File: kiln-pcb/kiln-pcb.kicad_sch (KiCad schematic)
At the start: 14 parts, among them J1 TFT, J2 TEMP, J3 ROTARY, J4 Relay, J5 Relay, J6 Relay, U1 WeMos_D1_mini

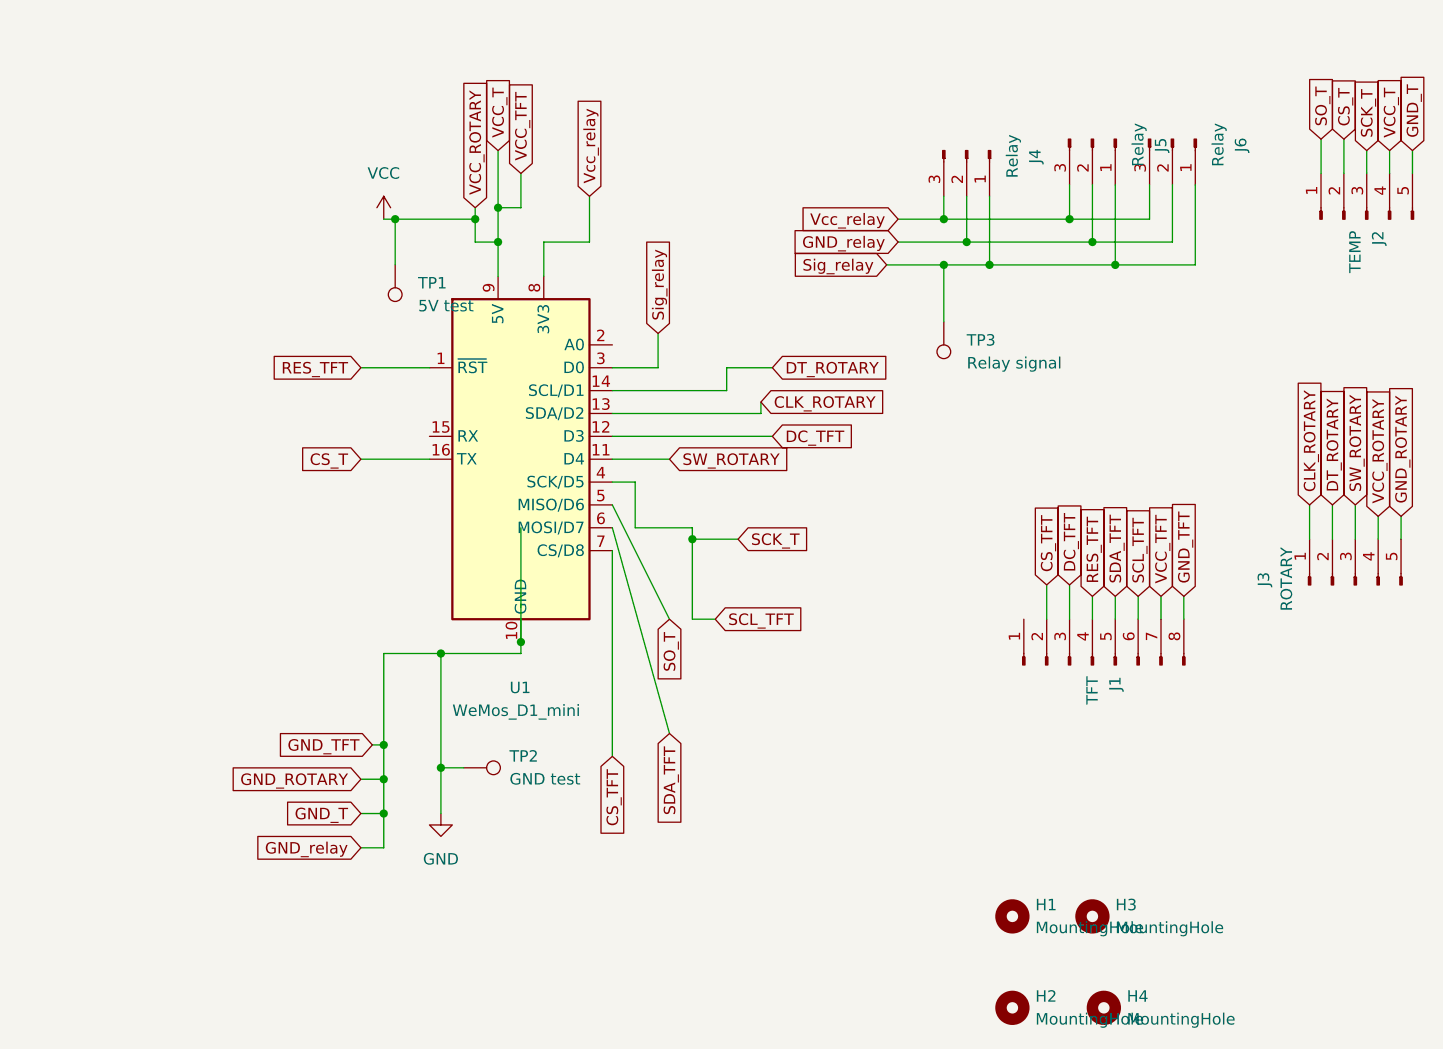
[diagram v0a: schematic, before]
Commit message: Basic README update
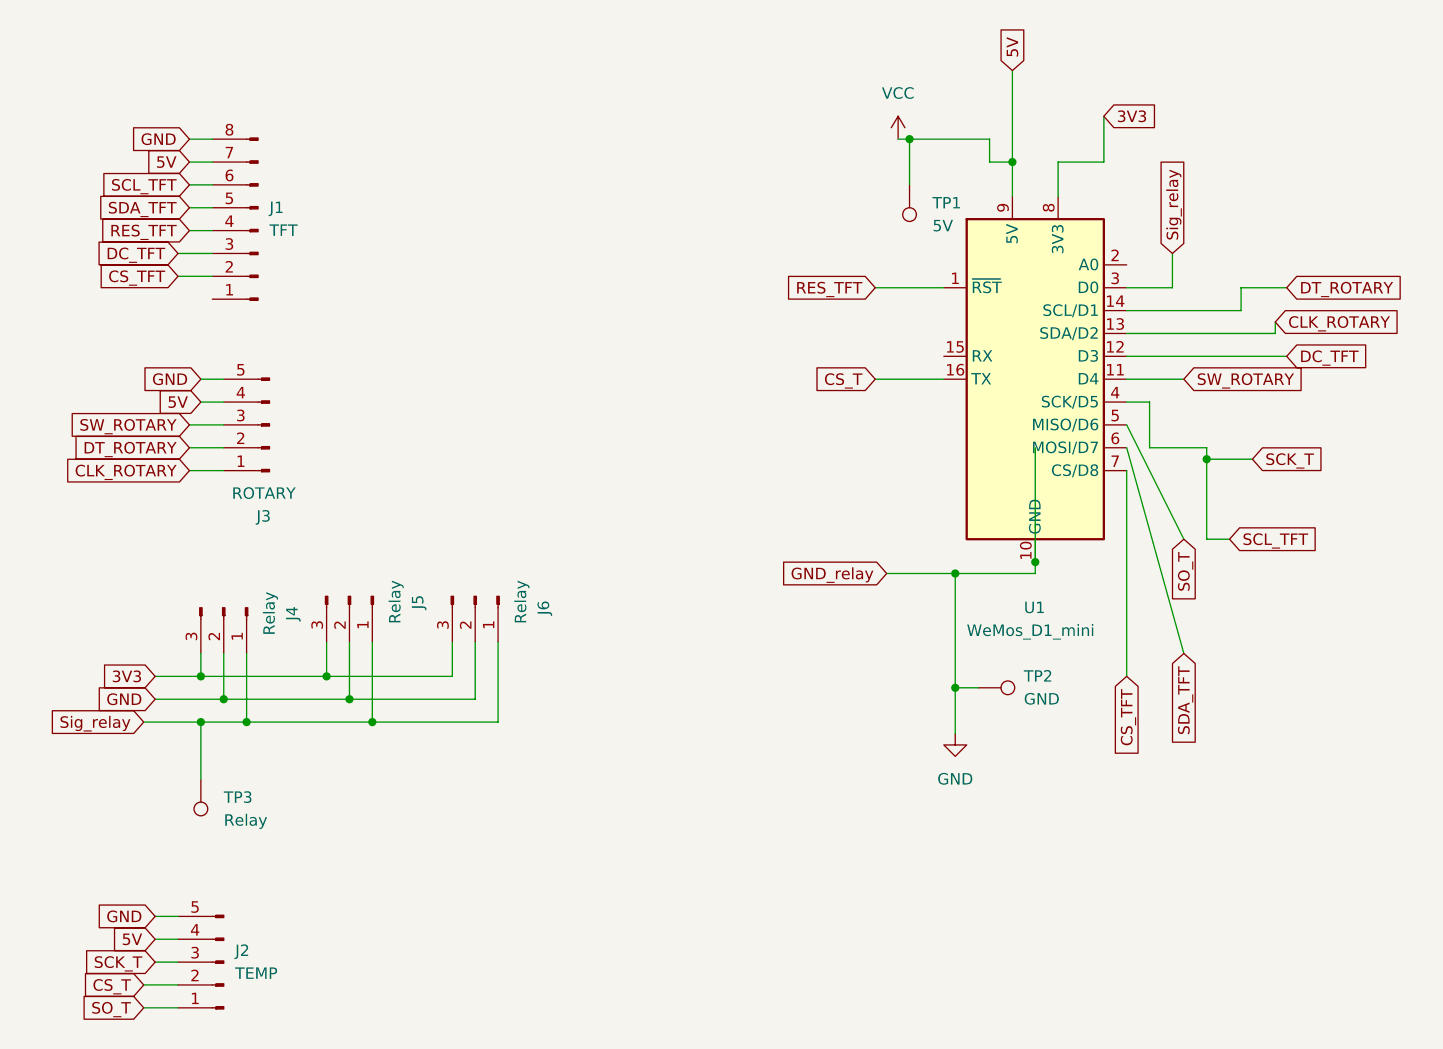
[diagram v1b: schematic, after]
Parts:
- removed H1, H2, H3, H4: MountingHole, MountingHole:MountingHole_3.2mm_M3_Pad_Via, symbol Mechanical:MountingHole
- TP1: value 5V test -> 5V
- TP2: value GND test -> GND
- TP3: value Relay signal -> Relay
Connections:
- net Vcc_relay renamed 3V3
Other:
- moved on the sheet: J1, J2, J3, J4, J5, J6, TP1, TP2, TP3, U1
